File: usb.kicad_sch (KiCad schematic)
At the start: 23 parts, among them IC2 USB Hub, J2 2-Port USB, J3 2-Port USB

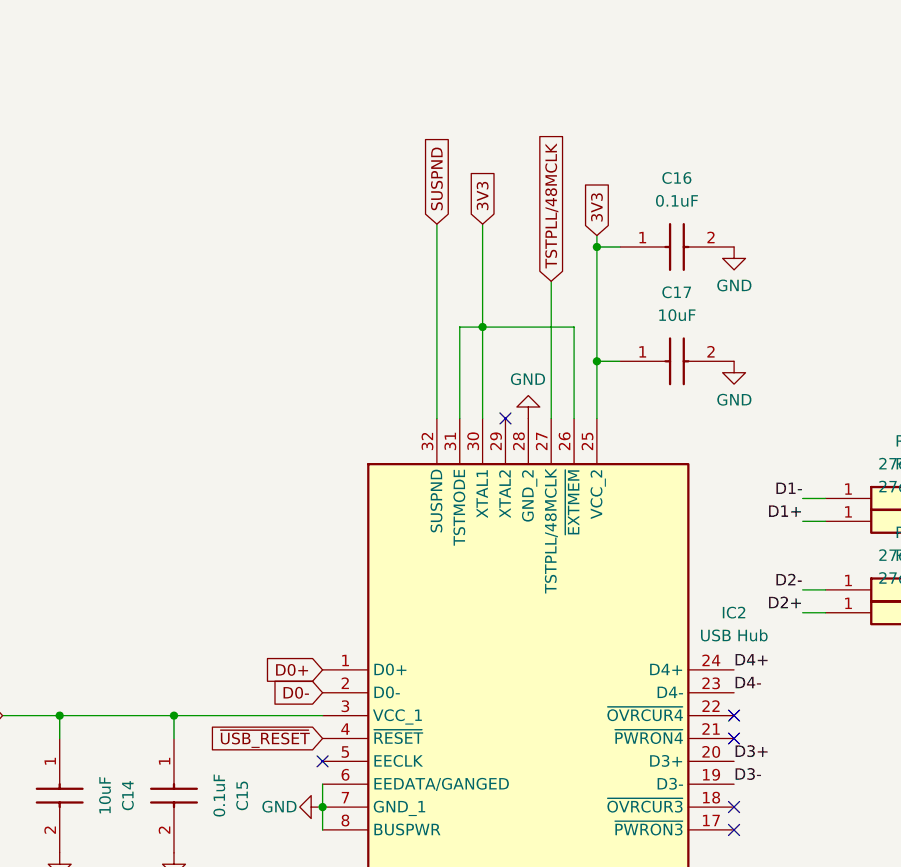
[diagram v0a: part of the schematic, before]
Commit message: USB stack changes
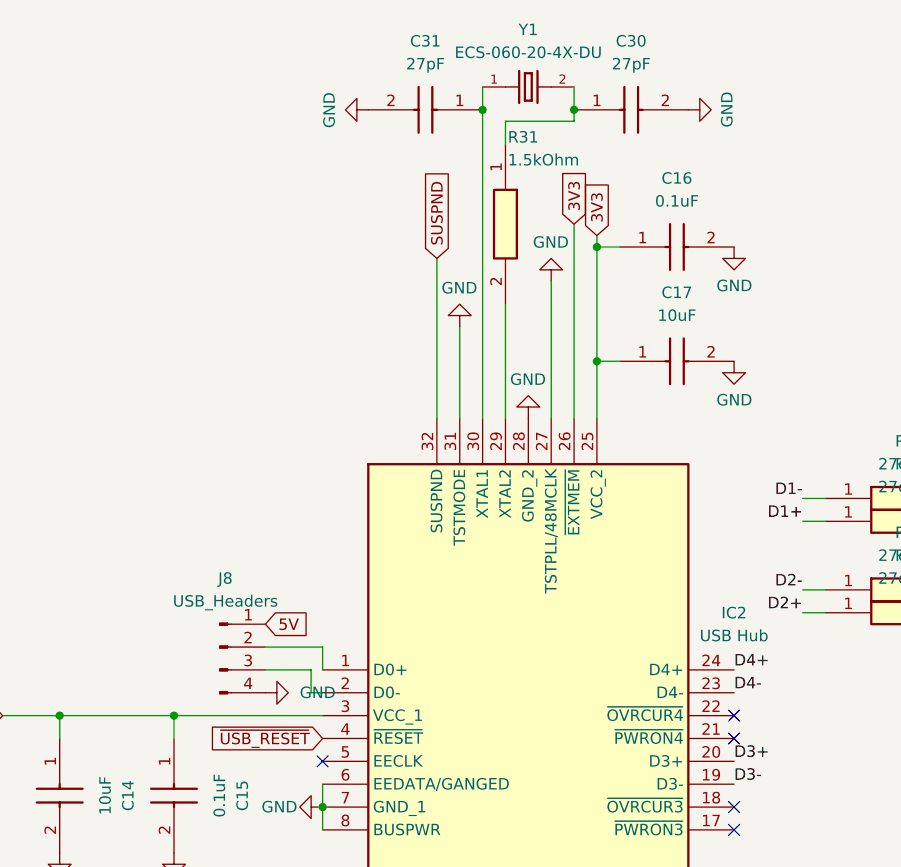
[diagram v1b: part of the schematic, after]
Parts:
- added C30, C31: 27pF, Capacitor_SMD:C_0805_2012Metric, symbol group127:0805Capacitor
- added J8: USB_Headers, Connector_PinHeader_2.54mm:PinHeader_1x04_P2.54mm_Vertical, symbol Connector:Conn_01x04_Pin
- added R31: 1.5kOhm, Resistor_SMD:R_0805_2012Metric, symbol group127:Resistor
- added Y1: ECS-060-20-4X-DU, group127:XTAL_ECS-160-20-4X, symbol group127:ECS-060-20-4X-DU
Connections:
- net TSTPLL/48MCLK is gone; now on net GND: IC2.27 (TSTPLL/48MCLK)
- net 3V3: no longer IC2.30 (XTAL1), IC2.31 (TSTMODE)
- net 5V: now also J8.1 (Pin_1)
- net GND: now also IC2.31 (TSTMODE), C30.2, C31.2, J8.4 (Pin_4)
- net at IC2.29 (XTAL2): now also R31.2
- net D0+: no longer names the net of IC2.1 (D0+)
- net D0+: now also J8.2 (Pin_2)
- net D0-: no longer names the net of IC2.2 (D0-)
- net D0-: now also J8.3 (Pin_3)
- new net: C30.1, R31.1, Y1.2
- new net: C31.1, IC2.30 (XTAL1), Y1.1
- no-connect marks 10 -> 9
